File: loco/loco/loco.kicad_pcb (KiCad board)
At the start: 2 copper layers, 3 parts, among them U1 STM32F030F4Px, U2 A4953_LJ

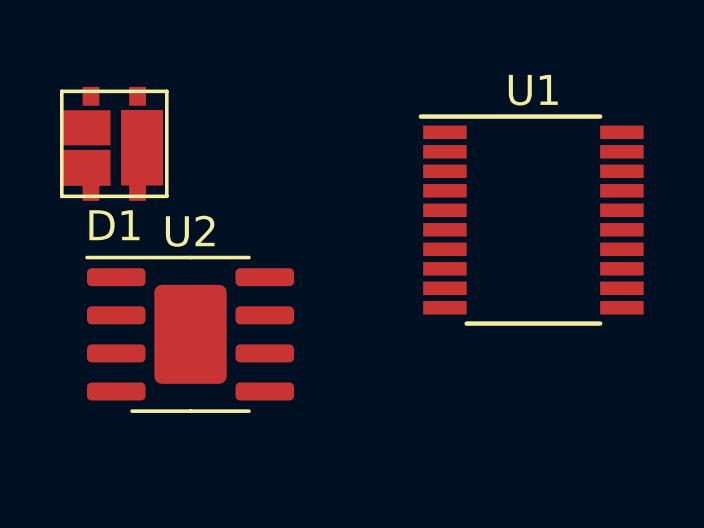
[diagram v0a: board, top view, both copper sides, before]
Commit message: Update
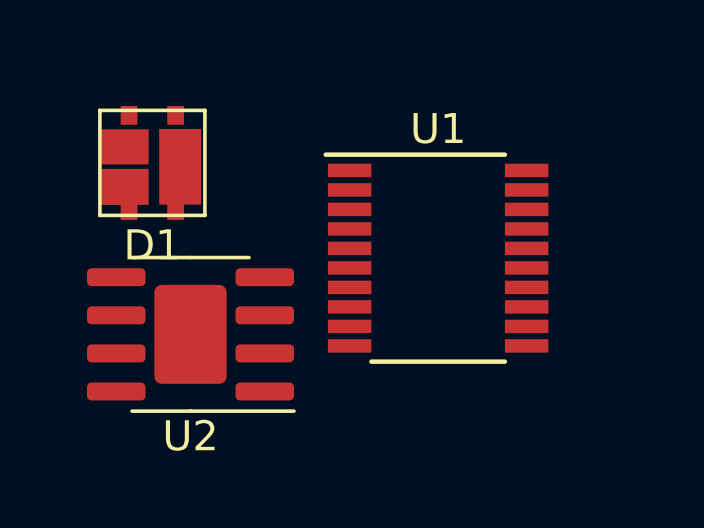
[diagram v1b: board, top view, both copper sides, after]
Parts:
- moved U1 3.42 mm to (128.9, 85.1)
- moved D1 1.42 mm to (119.4, 81.9)
- turned U2 to 180 degrees
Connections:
- net Net-(U1-Pad1) renamed /BOOT0
- net Net-(U1-Pad4) renamed /NRST
- net Net-(U2-Pad2) renamed /IN2
- net Net-(U2-Pad3) renamed /IN1
- net Net-(U2-Pad6) renamed /M1
- net Net-(U2-Pad8) renamed /M2
- U1 pad 16: Net-(U1-Pad16) -> /+3V3
- U1 pad 5: Net-(U1-Pad5) -> /+3V3
- U2 pad 1: Net-(U2-Pad1) -> GND
- U2 pad 5: Net-(U2-Pad5) -> /27V
- U2 pad 9: Net-(U2-Pad9) -> GND
